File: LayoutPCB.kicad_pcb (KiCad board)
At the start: 2 copper layers, 59.2 x 48.9 mm, 37 parts, among them J1 USB_B_Micro, J2 Conn_01x01_Female, J3 Conn_01x01_Female, J4 Conn_01x01_Female, J5 Conn_01x01_Female, J6 Conn_01x01_Female, J7 Conn_01x01_Female, U1 TP4056, U2 DW01, U3 FS8205A

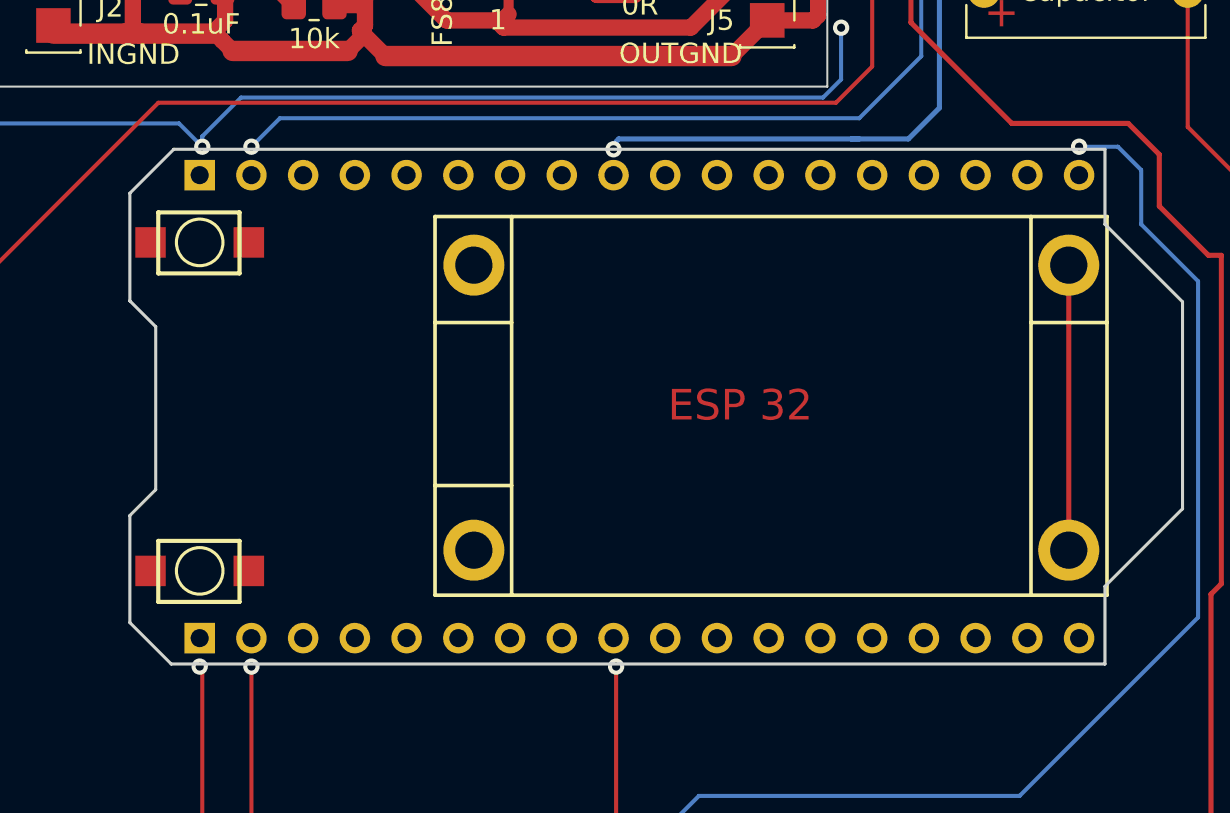
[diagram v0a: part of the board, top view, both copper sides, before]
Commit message: Gerando os arquivos
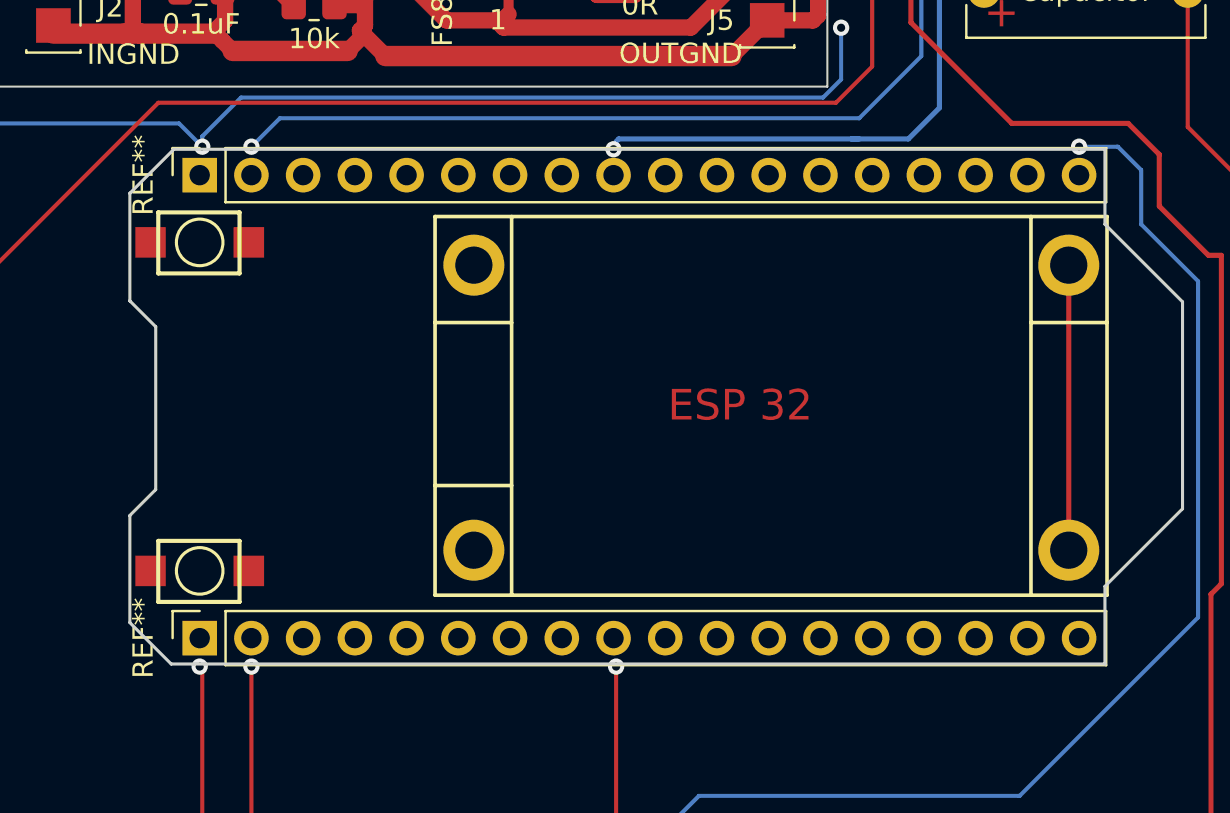
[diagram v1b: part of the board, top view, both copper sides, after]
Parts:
- added REF**: PinSocket_1x18_P2.54mm_Vertical, Connector_PinSocket_2.54mm:PinSocket_1x18_P2.54mm_Vertical, F.Cu at (76.3, 78.9)
- added REF**: PinSocket_1x18_P2.54mm_Vertical, Connector_PinSocket_2.54mm:PinSocket_1x18_P2.54mm_Vertical, F.Cu at (76.3, 101.6)
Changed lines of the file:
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@@
       (sketchpadsonfab false)
       (subtractmaskfromsilk false)
-      (outputformat 5)
-      (mirror true)
-      (drillshape 2)
+      (outputformat 1)
+      (mirror false)
+      (drillshape 0)
       (scaleselection 1)
       (outputdirectory "out/")
@@
   (net 17 "/G1")
   (net 18 "unconnected-(J1-Pad6)")
+  (footprint "Connector_PinSocket_2.54mm:PinSocket_1x18_P2.54mm_Vertical" (layer "F.Cu")
+    (at 76.327 78.867 90)
+    (descr "Through hole straight socket strip, 1x18, 2.54mm pitch, single row (from Kicad 4.0.7), script generated")
+    (tags "Through hole socket strip THT 1x18 2.54mm single row")
+    (attr through_hole)
+    (fp_text reference "REF**" (at 0 -2.77 90) (layer "F.SilkS")
+      (effects (font (size 1 1) (thickness 0.15)))
+    )
+    (fp_text value "PinSocket_1x18_P2.54mm_Vertical" (at 0 45.95 90) (layer "F.Fab")
+      (effects (font (size 1 1) (thickness 0.15)))
+    )
+    (fp_text user "${REFERENCE}" (at 0 21.59) (layer "F.Fab")
+      (effects (font (size 1 1) (thickness 0.15)))
+    )
+    (fp_line (start -1.33 1.27) (end 1.33 1.27) (layer "F.SilkS") (width 0.12))
+    (fp_line (start -1.33 1.27) (end -1.33 44.51) (layer "F.SilkS") (width 0.12))
+    (fp_line (start 0 -1.33) (end 1.33 -1.33) (layer "F.SilkS") (width 0.12))
+    (fp_line (start -1.33 44.51) (end 1.33 44.51) (layer "F.SilkS") (width 0.12))
+    (fp_line (start 1.33 -1.33) (end 1.33 0) (layer "F.SilkS") (width 0.12))
+    (fp_line (start 1.33 1.27) (end 1.33 44.51) (layer "F.SilkS") (width 0.12))
+    (fp_line (start 1.75 44.95) (end -1.8 44.95) (layer "F.CrtYd") (width 0.05))
+    (fp_line (start -1.8 44.95) (end -1.8 -1.8) (layer "F.CrtYd") (width 0.05))
+    (fp_line (start -1.8 -1.8) (end 1.75 -1.8) (layer "F.CrtYd") (width 0.05))
+    (fp_line (start 1.75 -1.8) (end 1.75 44.95) (layer "F.CrtYd") (width 0.05))
+    (fp_line (start 0.635 -1.27) (end 1.27 -0.635) (layer "F.Fab") (width 0.1))
+    (fp_line (start 1.27 -0.635) (end 1.27 44.45) (layer "F.Fab") (width 0.1))
+    (fp_line (start -1.27 44.45) (end -1.27 -1.27) (layer "F.Fab") (width 0.1))
+    (fp_line (start -1.27 -1.27) (end 0.635 -1.27) (layer "F.Fab") (width 0.1))
+    (fp_line (start 1.27 44.45) (end -1.27 44.45) (layer "F.Fab") (width 0.1))
+    (pad "1" thru_hole rect (at 0 0 90) (size 1.7 1.7) (drill 1) (layers *.Cu *.Mask))
+    (pad "2" thru_hole oval (at 0 2.54 90) (size 1.7 1.7) (drill 1) (layers *.Cu *.Mask))
+    (pad "3" thru_hole oval (at 0 5.08 90) (size 1.7 1.7) (drill 1) (layers *.Cu *.Mask))
+    (pad "4" thru_hole oval (at 0 7.62 90) (size 1.7 1.7) (drill 1) (layers *.Cu *.Mask))
+    (pad "5" thru_hole oval (at 0 10.16 90) (size 1.7 1.7) (drill 1) (layers *.Cu *.Mask))
+    (pad "6" thru_hole oval (at 0 12.7 90) (size 1.7 1.7) (drill 1) (layers *.Cu *.Mask))
+    (pad "7" thru_hole oval (at 0 15.24 90) (size 1.7 1.7) (drill 1) (layers *.Cu *.Mask))
+    (pad "8" thru_hole oval (at 0 17.78 90) (size 1.7 1.7) (drill 1) (layers *.Cu *.Mask))
+    (pad "9" thru_hole oval (at 0 20.32 90) (size 1.7 1.7) (drill 1) (layers *.Cu *.Mask))
+    (pad "10" thru_hole oval (at 0 22.86 90) (size 1.7 1.7) (drill 1) (layers *.Cu *.Mask))
+    (pad "11" thru_hole oval (at 0 25.4 90) (size 1.7 1.7) (drill 1) (layers *.Cu *.Mask))
+    (pad "12" thru_hole oval (at 0 27.94 90) (size 1.7 1.7) (drill 1) (layers *.Cu *.Mask))
+    (pad "13" thru_hole oval (at 0 30.48 90) (size 1.7 1.7) (drill 1) (layers *.Cu *.Mask))
+    (pad "14" thru_hole oval (at 0 33.02 90) (size 1.7 1.7) (drill 1) (layers *.Cu *.Mask))
+    (pad "15" thru_hole oval (at 0 35.56 90) (size 1.7 1.7) (drill 1) (layers *.Cu *.Mask))
+    (pad "16" thru_hole oval (at 0 38.1 90) (size 1.7 1.7) (drill 1) (layers *.Cu *.Mask))
+    (pad "17" thru_hole oval (at 0 40.64 90) (size 1.7 1.7) (drill 1) (layers *.Cu *.Mask))
+    (pad "18" thru_hole oval (at 0 43.18 90) (size 1.7 1.7) (drill 1) (layers *.Cu *.Mask))
+    (model "${KICAD6_3DMODEL_DIR}/Connector_PinSocket_2.54mm.3dshapes/PinSocket_1x18_P2.54mm_Vertical.wrl"
+      (offset (xyz 0 0 0))
+      (scale (xyz 1 1 1))
+      (rotate (xyz 0 0 0))
+    )
+  )
+  (footprint "Connector_PinSocket_2.54mm:PinSocket_1x18_P2.54mm_Vertical" (layer "F.Cu")
+    (at 76.327 101.6 90)
+    (descr "Through hole straight socket strip, 1x18, 2.54mm pitch, single row (from Kicad 4.0.7), script generated")
+    (tags "Through hole socket strip THT 1x18 2.54mm single row")
+    (attr through_hole)
+    (fp_text reference "REF**" (at 0 -2.77 90) (layer "F.SilkS")
+      (effects (font (size 1 1) (thickness 0.15)))
+    )
+    (fp_text value "PinSocket_1x18_P2.54mm_Vertical" (at 0 45.95 90) (layer "F.Fab")
+      (effects (font (size 1 1) (thickness 0.15)))
+    )
+    (fp_text user "${REFERENCE}" (at 0 21.59) (layer "F.Fab")
+      (effects (font (size 1 1) (thickness 0.15)))
+    )
+    (fp_line (start -1.33 44.51) (end 1.33 44.51) (layer "F.SilkS") (width 0.12))
+    (fp_line (start 1.33 -1.33) (end 1.33 0) (layer "F.SilkS") (width 0.12))
+    (fp_line (start -1.33 1.27) (end -1.33 44.51) (layer "F.SilkS") (width 0.12))
+    (fp_line (start 0 -1.33) (end 1.33 -1.33) (layer "F.SilkS") (width 0.12))
+    (fp_line (start 1.33 1.27) (end 1.33 44.51) (layer "F.SilkS") (width 0.12))
+    (fp_line (start -1.33 1.27) (end 1.33 1.27) (layer "F.SilkS") (width 0.12))
+    (fp_line (start -1.8 44.95) (end -1.8 -1.8) (layer "F.CrtYd") (width 0.05))
+    (fp_line (start 1.75 -1.8) (end 1.75 44.95) (layer "F.CrtYd") (width 0.05))
+    (fp_line (start 1.75 44.95) (end -1.8 44.95) (layer "F.CrtYd") (width 0.05))
+    (fp_line (start -1.8 -1.8) (end 1.75 -1.8) (layer "F.CrtYd") (width 0.05))
+    (fp_line (start -1.27 -1.27) (end 0.635 -1.27) (layer "F.Fab") (width 0.1))
+    (fp_line (start 0.635 -1.27) (end 1.27 -0.635) (layer "F.Fab") (width 0.1))
+    (fp_line (start 1.27 -0.635) (end 1.27 44.45) (layer "F.Fab") (width 0.1))
+    (fp_line (start 1.27 44.45) (end -1.27 44.45) (layer "F.Fab") (width 0.1))
+    (fp_line (start -1.27 44.45) (end -1.27 -1.27) (layer "F.Fab") (width 0.1))
+    (pad "1" thru_hole rect (at 0 0 90) (size 1.7 1.7) (drill 1) (layers *.Cu *.Mask))
+    (pad "2" thru_hole oval (at 0 2.54 90) (size 1.7 1.7) (drill 1) (layers *.Cu *.Mask))
+    (pad "3" thru_hole oval (at 0 5.08 90) (size 1.7 1.7) (drill 1) (layers *.Cu *.Mask))
+    (pad "4" thru_hole oval (at 0 7.62 90) (size 1.7 1.7) (drill 1) (layers *.Cu *.Mask))
+    (pad "5" thru_hole oval (at 0 10.16 90) (size 1.7 1.7) (drill 1) (layers *.Cu *.Mask))
+    (pad "6" thru_hole oval (at 0 12.7 90) (size 1.7 1.7) (drill 1) (layers *.Cu *.Mask))
+    (pad "7" thru_hole oval (at 0 15.24 90) (size 1.7 1.7) (drill 1) (layers *.Cu *.Mask))
+    (pad "8" thru_hole oval (at 0 17.78 90) (size 1.7 1.7) (drill 1) (layers *.Cu *.Mask))
+    (pad "9" thru_hole oval (at 0 20.32 90) (size 1.7 1.7) (drill 1) (layers *.Cu *.Mask))
+    (pad "10" thru_hole oval (at 0 22.86 90) (size 1.7 1.7) (drill 1) (layers *.Cu *.Mask))
+    (pad "11" thru_hole oval (at 0 25.4 90) (size 1.7 1.7) (drill 1) (layers *.Cu *.Mask))
+    (pad "12" thru_hole oval (at 0 27.94 90) (size 1.7 1.7) (drill 1) (layers *.Cu *.Mask))
+    (pad "13" thru_hole oval (at 0 30.48 90) (size 1.7 1.7) (drill 1) (layers *.Cu *.Mask))
+    (pad "14" thru_hole oval (at 0 33.02 90) (size 1.7 1.7) (drill 1) (layers *.Cu *.Mask))
+    (pad "15" thru_hole oval (at 0 35.56 90) (size 1.7 1.7) (drill 1) (layers *.Cu *.Mask))
+    (pad "16" thru_hole oval (at 0 38.1 90) (size 1.7 1.7) (drill 1) (layers *.Cu *.Mask))
+    (pad "17" thru_hole oval (at 0 40.64 90) (size 1.7 1.7) (drill 1) (layers *.Cu *.Mask))
+    (pad "18" thru_hole oval (at 0 43.18 90) (size 1.7 1.7) (drill 1) (layers *.Cu *.Mask))
+    (model "${KICAD6_3DMODEL_DIR}/Connector_PinSocket_2.54mm.3dshapes/PinSocket_1x18_P2.54mm_Vertical.wrl"
+      (offset (xyz 0 0 0))
+      (scale (xyz 1 1 1))
+      (rotate (xyz 0 0 0))
+    )
+  )
   (footprint "Connector_PinSocket_2.54mm:PinSocket_1x01_P2.54mm_Vertical" (layer "F.Cu")
     (at 104.1948 71.269)
